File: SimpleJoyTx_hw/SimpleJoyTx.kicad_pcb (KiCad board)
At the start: 2 copper layers, 108 x 66 mm, 88 parts, among them J1 Joystick, J2 Joystick, Q1 2N7002, SW1 IT-1187A, SW2 DIPx8, SW3 SWITCH, SW4 IT-1187A, SW5 IT-1187A, SW6 IT-1187A, SW7 IT-1187A, SW8 IT-1187A, U1 USBLC6, U2 BT_HC05

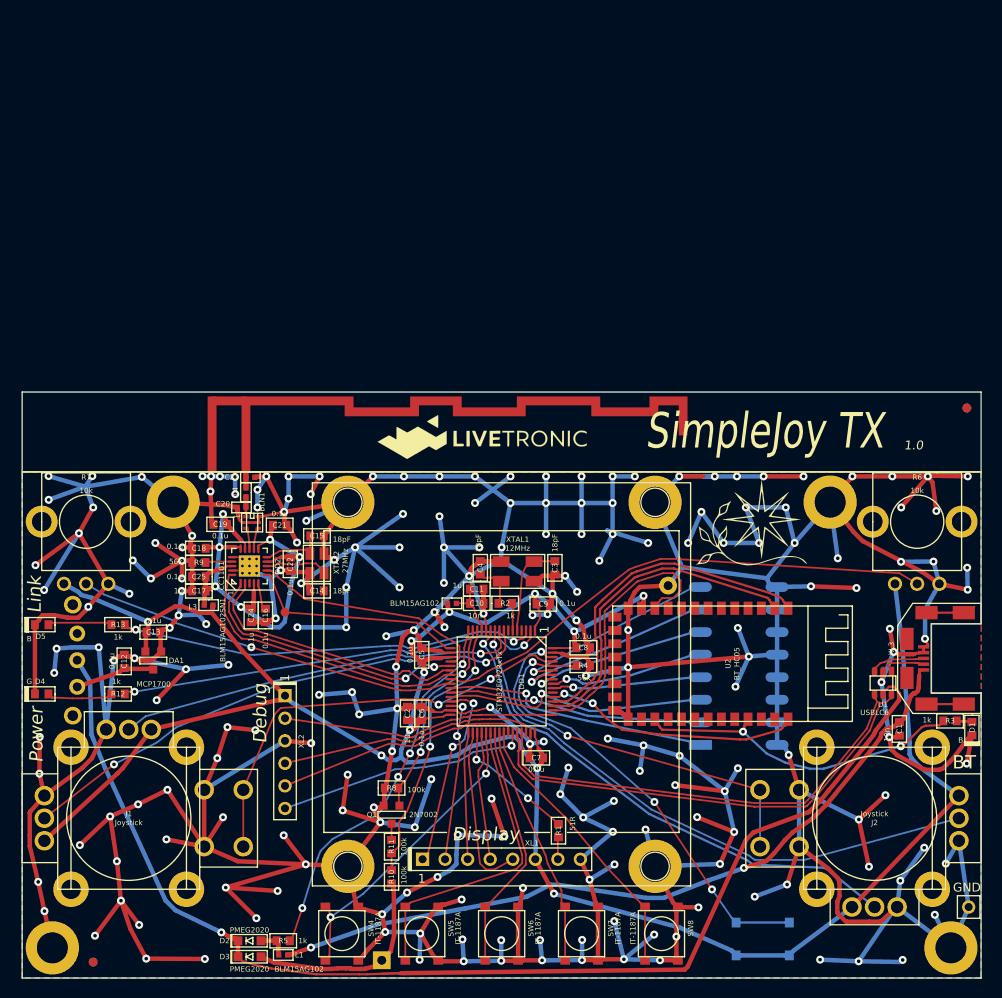
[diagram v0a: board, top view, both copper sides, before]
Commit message: Proceeding
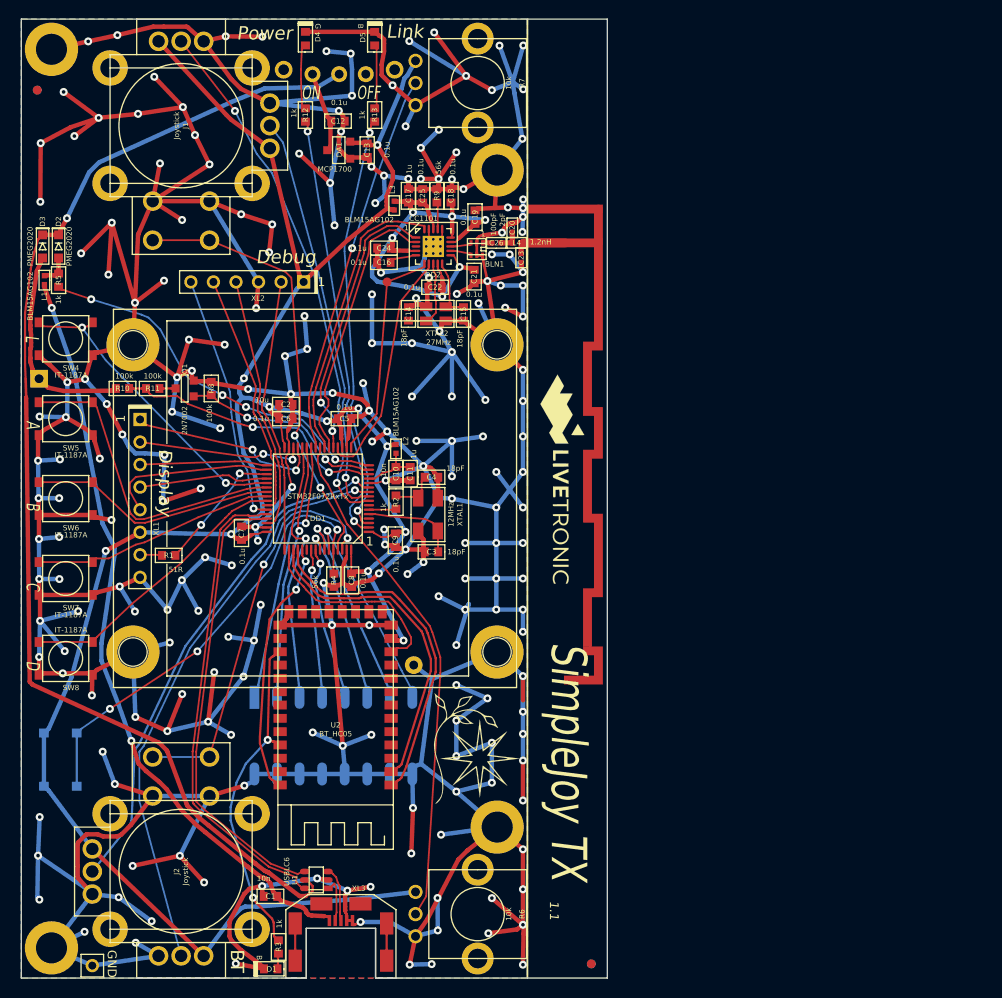
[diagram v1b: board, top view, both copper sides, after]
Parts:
- added C26: 100pF, Capacitors:CAP_0402, F.Cu at (163.4, 32.2)
- C20: value * -> 2pF
- C23: value * -> DoNotMount
- DA1: footprint SOT:SOT23-3 -> SOT:SOT23-3A
- L3: value BLM15AG102SN1 -> BLM15AG102
- L4: value * -> 1.2nH
- XL1: value PLS-8 -> PBS-8
- moved HOLE3 101.3 mm to (113.3, 111.6), turned to 270 degrees
- moved HOLE2 101.2 mm to (113.3, 10.4), turned to 270 degrees
- moved XL4 98.9 mm to (117.9, 113.6), turned to 270 degrees
- moved RP1 98.4 mm to (111.7, 15.0), turned to 270 degrees
- moved RP2 98.4 mm to (111.7, 15.0), turned to 270 degrees
- moved D1 83.5 mm to (138.0, 114.0), turned to 180 degrees
- moved D3 83.3 mm to (112.3, 32.6), turned to 270 degrees
- moved SW1 81.6 mm to (114.3, 90.4), turned to 90 degrees
- moved D2 81.1 mm to (114.1, 32.6), turned to 270 degrees
- moved L1 80.6 mm to (112.5, 36.4), turned to 270 degrees
- moved R3 79.8 mm to (138.9, 111.5), turned to 90 degrees
- moved D4 79.6 mm to (141.9, 9.20), turned to 90 degrees
- moved R5 78.6 mm to (114.1, 36.4), turned to 270 degrees
- moved J2 78.3 mm to (127.9, 103.0), turned to 270 degrees
- moved J1 78.2 mm to (127.9, 19.0), turned to 90 degrees
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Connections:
- BLN1 pad 1: /ANT1 -> Net-(BLN1-Pad1)
- R10 pad 1: +BATT -> /BAT_MEAS
- R10 pad 2: /BAT_MEAS -> +BATT
- R11 pad 1: /BAT_MEAS -> Net-(Q1-Pad3)
- R11 pad 2: Net-(Q1-Pad3) -> /BAT_MEAS
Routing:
- net /BT_RESET: track 30.2 -> 23.1 mm
- net GND: track 1270.7 -> 1267.0 mm
- net VCC: track 60.3 -> 63.1 mm
- net +3.3V: track 269.5 -> 270.8 mm
- net Net-(BLN1-Pad1): track 0.00 -> 1.31 mm
- net Net-(Q1-Pad3): track 1.83 -> 3.10 mm
- net /PWR_UNST_ALWAYS: track 135.8 -> 136.8 mm
- net /ANT2: track 9.45 -> 10.0 mm
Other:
- board size 108 x 66 mm -> 66 x 108 mm
- board text added: "1.1"
- board text added: "A"
- board text added: "C"
- board text added: "D"
- board text added: "L"
- board text added: "OFF"
- board text added: "ON"
- board text removed: "1.0"
